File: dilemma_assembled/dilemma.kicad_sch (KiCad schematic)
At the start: 103 parts, among them J1 USB_C_Receptacle_USB2.0, J102 NA_serial, J105 NA_Conn_01x04_Female, J113 Cirque, J2 NA_Conn_01x03_Female, J3 NA_GC9A01, J5 Conn_01x02, SW1 SW_Push, SW101 NA_SW_Push, SW102 NA_SW_Push, SW103 NA_SW_Push, SW104 NA_SW_Push, SW105 NA_SW_Push, SW106 NA_SW_Push, SW107 NA_SW_Push, SW108 NA_SW_Push, SW109 NA_SW_Push, SW110 NA_SW_SPST, SW112 NA_SW_Push, SW113 NA_SW_Push, SW114 NA_SW_Push, SW115 NA_SW_Push, SW116 NA_SW_Push, SW117 NA_SW_Push, SW118 NA_SW_Push, SW119 NA_SW_Push, SW2 SW_Push, SW3001 NA_SW_Push, SW3002 NA_RotaryEncoder_Switch, U1 RP2040, U2 W25Q128JVS, U3 XC6210B332MR-G, U4 USBLC6-2P6, Y1 Crystal_GND24

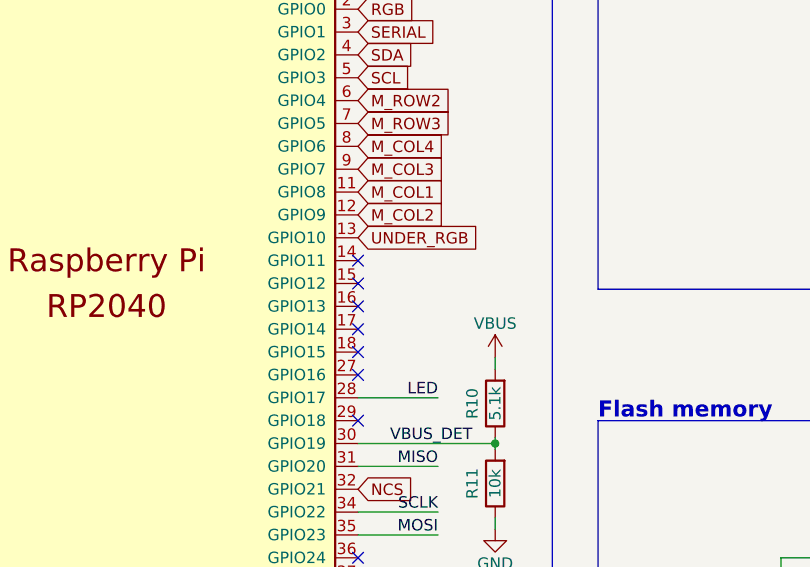
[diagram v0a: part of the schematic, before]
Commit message: routing
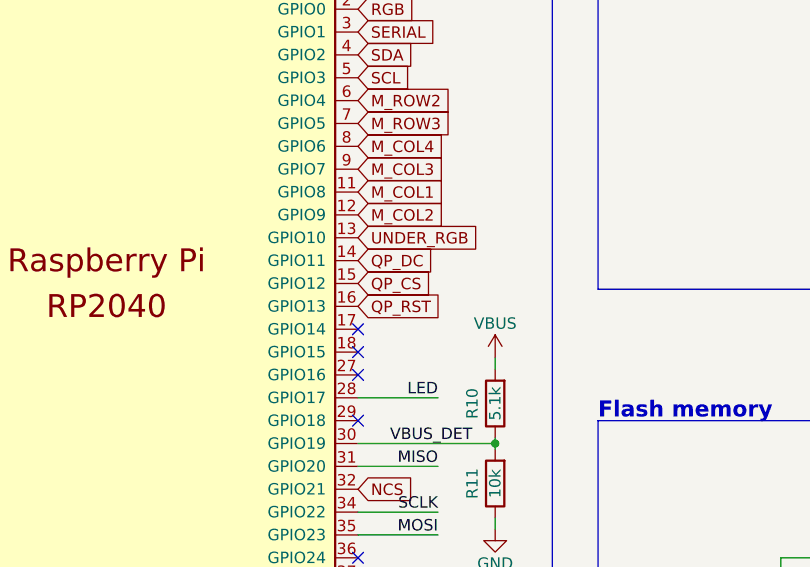
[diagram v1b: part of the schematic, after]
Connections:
- net QP_CS: now also U1.15 (GPIO12)
- net QP_DC: now also U1.14 (GPIO11)
- net QP_RST: now also U1.16 (GPIO13)
- no-connect marks 19 -> 16
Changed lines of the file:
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@@
   (no_connect (at 182.88 121.92))
   (no_connect (at 182.88 104.14))
-  (no_connect (at 182.88 86.36))
   (no_connect (at 265.43 176.53))
   (no_connect (at 50.8 64.77))
   (no_connect (at 50.8 67.31))
   (no_connect (at 342.265 45.72))
-  (no_connect (at 182.88 88.9))
-  (no_connect (at 182.88 91.44))
   (no_connect (at 182.88 93.98))
   (no_connect (at 182.88 96.52))
@@
     )
   )
+  (global_label "QP_CS" (shape input) (at 182.88 88.9 0) (fields_autoplaced)
+    (effects (font (size 1.27 1.27)) (justify left))
+    (property "Intersheet References" "${INTERSHEET_REFS}" (id 0) (at 191.3407 88.8206 0)
+      (effects (font (size 1.27 1.27)) (justify left) hide)
+    )
+  )
   (global_label "M_ROW3" (shape input) (at 182.88 71.12 0)
     (effects (font (size 1.27 1.27)) (justify left))
@@
     )
   )
+  (global_label "QP_RST" (shape input) (at 182.88 91.44 0) (fields_autoplaced)
+    (effects (font (size 1.27 1.27)) (justify left))
+    (property "Intersheet References" "${INTERSHEET_REFS}" (id 0) (at 192.3083 91.3606 0)
+      (effects (font (size 1.27 1.27)) (justify left) hide)
+    )
+  )
   (global_label "M_COL2" (shape input) (at 93.98 213.36 90)
     (effects (font (size 1.27 1.27)) (justify left))
@@
     )
   )
+  (global_label "QP_DC" (shape input) (at 182.88 86.36 0) (fields_autoplaced)
+    (effects (font (size 1.27 1.27)) (justify left))
+    (property "Intersheet References" "${INTERSHEET_REFS}" (id 0) (at 191.4012 86.2806 0)
+      (effects (font (size 1.27 1.27)) (justify left) hide)
+    )
+  )
